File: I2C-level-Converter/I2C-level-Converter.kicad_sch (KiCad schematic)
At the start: 17 parts, among them J3 DF13-4P-1.25V(21), J4 LABEL, U1 PCA9306D,118, U2 MIC5365-3.3YC5

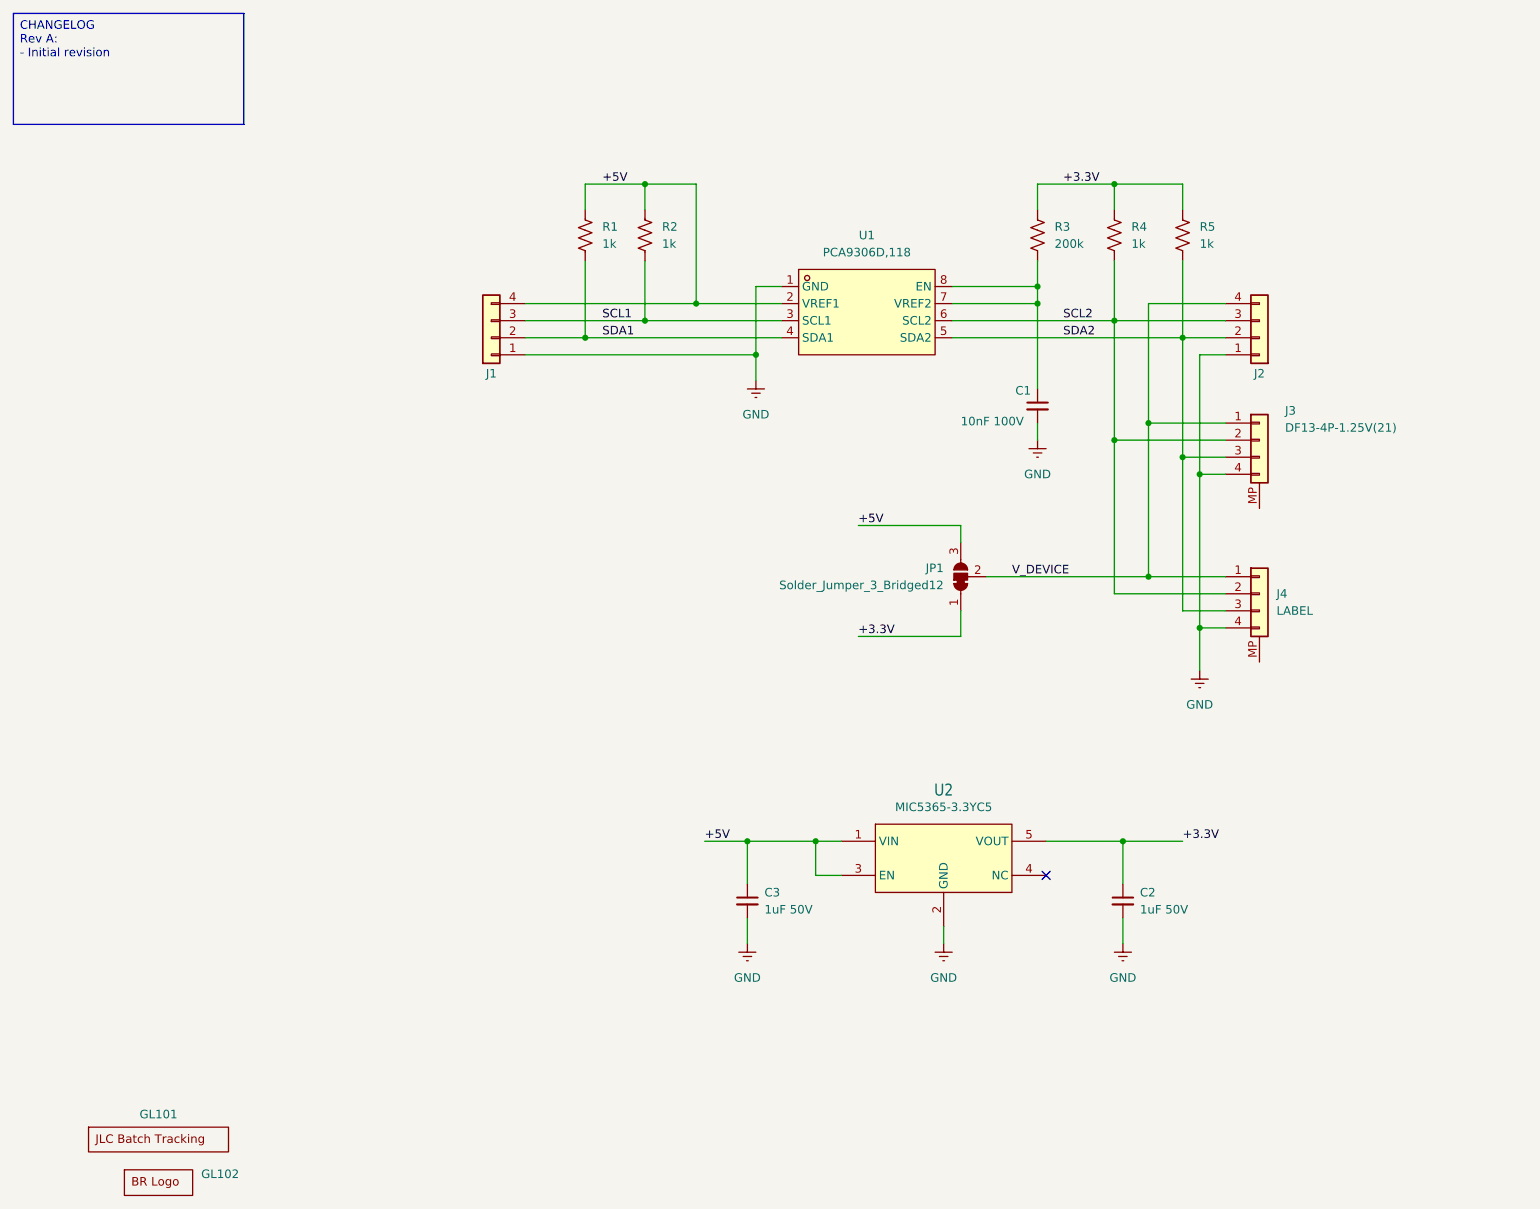
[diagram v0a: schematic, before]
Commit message: finish
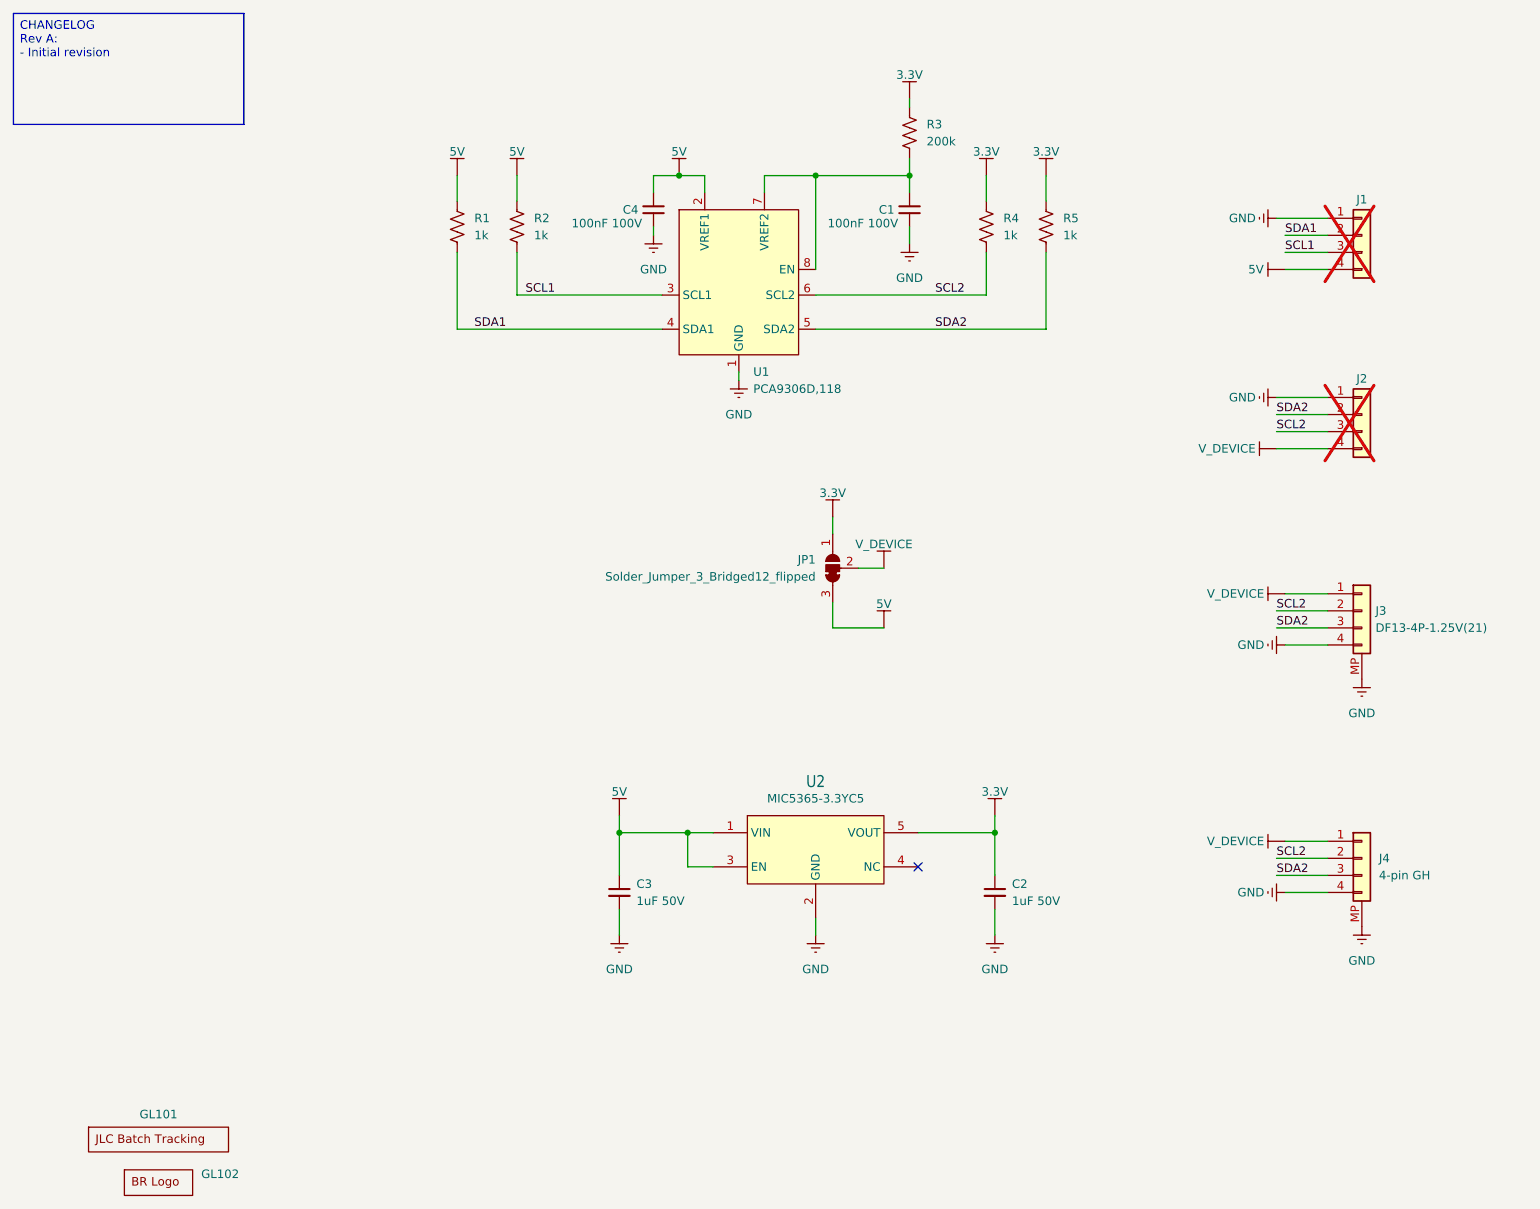
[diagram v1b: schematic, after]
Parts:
- added C4: 100nF 100V, BR_Passives:C_0603_1608Metric-minimized, symbol BR_Capacitors_0603:C_0603_100nF_100V_X7R_AEC-Q200
- C1: value 10nF 100V -> 100nF 100V; symbol BR_Capacitors_0603:C_0603_10nF_100V_X7R_10% -> BR_Capacitors_0603:C_0603_100nF_100V_X7R_AEC-Q200; BRE Number BRE-001155 -> BRE-000034; JLCPCB Part Num C84709 -> C161117; Manufacturer Samsung Electro-Mechanics -> Murata Electronics; Manufacturer Part Num CL10B103KC8NNNC -> GCJ188R72A104KA01D; Supplier 1 JLCPCB -> DigiKey; Supplier 2 (none) -> Mouser; Supplier 3 (none) -> JLCPCB; Supplier Part Num 1 C84709 -> 490-13420-1-ND; Supplier Part Num 2 (none) -> 81-GCJ188R72A104KA1D; Supplier Part Num 3 (none) -> C161117
- J1: now not fitted
- J2: value ~ -> 4-pin header; now not fitted
- J4: value LABEL -> 4-pin GH
- JP1: value Solder_Jumper_3_Bridged12 -> Solder_Jumper_3_Bridged12_flipped; footprint BR_Virtual_Parts:SolderJumper-3_P1.3mm_Open_Pad1.0x1.5mm -> BR_Virtual_Parts:SolderJumper-3_P1.3mm_Open_Pad1.0x1.5mm_paste; symbol BR_Virtual_Parts:Solder_Jumper_3_Bridged12-Jumper_small -> BR_Virtual_Parts:Solder_Jumper_3_Bridged12-Jumper_flipped
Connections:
- net GND: now also J3.MP, J4.MP, C4.2
- net +3.3V renamed 3.3V
- net +5V renamed 5V
- net 5V: now also C4.1
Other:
- title: (none) -> I2C Level Converter
- moved on the sheet: C1, C2, C3, J3, J4, JP1, R1, R2, R3, R4, R5, U2
